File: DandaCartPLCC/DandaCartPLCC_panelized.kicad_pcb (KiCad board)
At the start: 2 copper layers, 93 x 96 mm, 18 parts, among them P1 DAN_CART_EDGE, P2 DAN_CART_EDGE, P3 DAN_CART_EDGE, P4 DAN_CART_EDGE, P5 DAN_CART_EDGE, P6 DAN_CART_EDGE, U1 SST39SF040, U2 SST39SF040, U3 SST39SF040, U4 SST39SF040, U5 SST39SF040, U6 SST39SF040

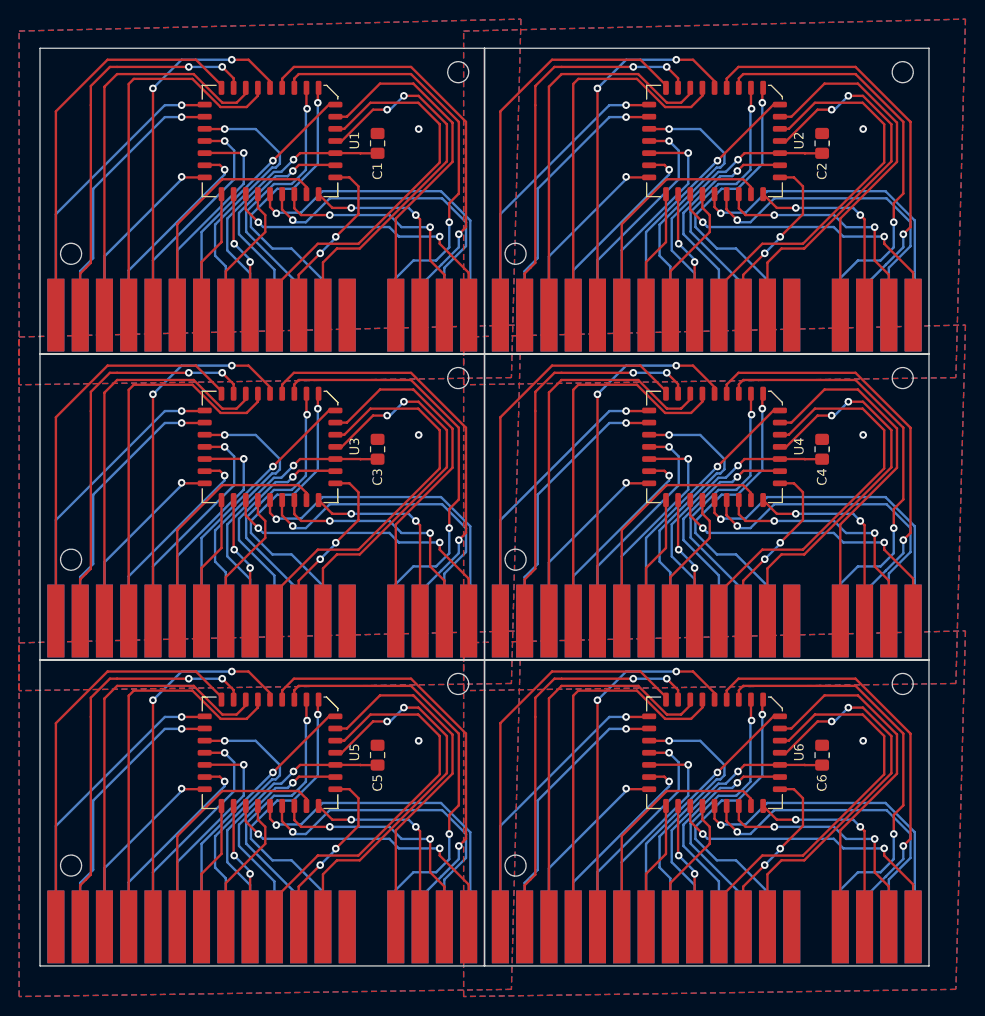
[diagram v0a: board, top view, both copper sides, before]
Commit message: Add files via upload
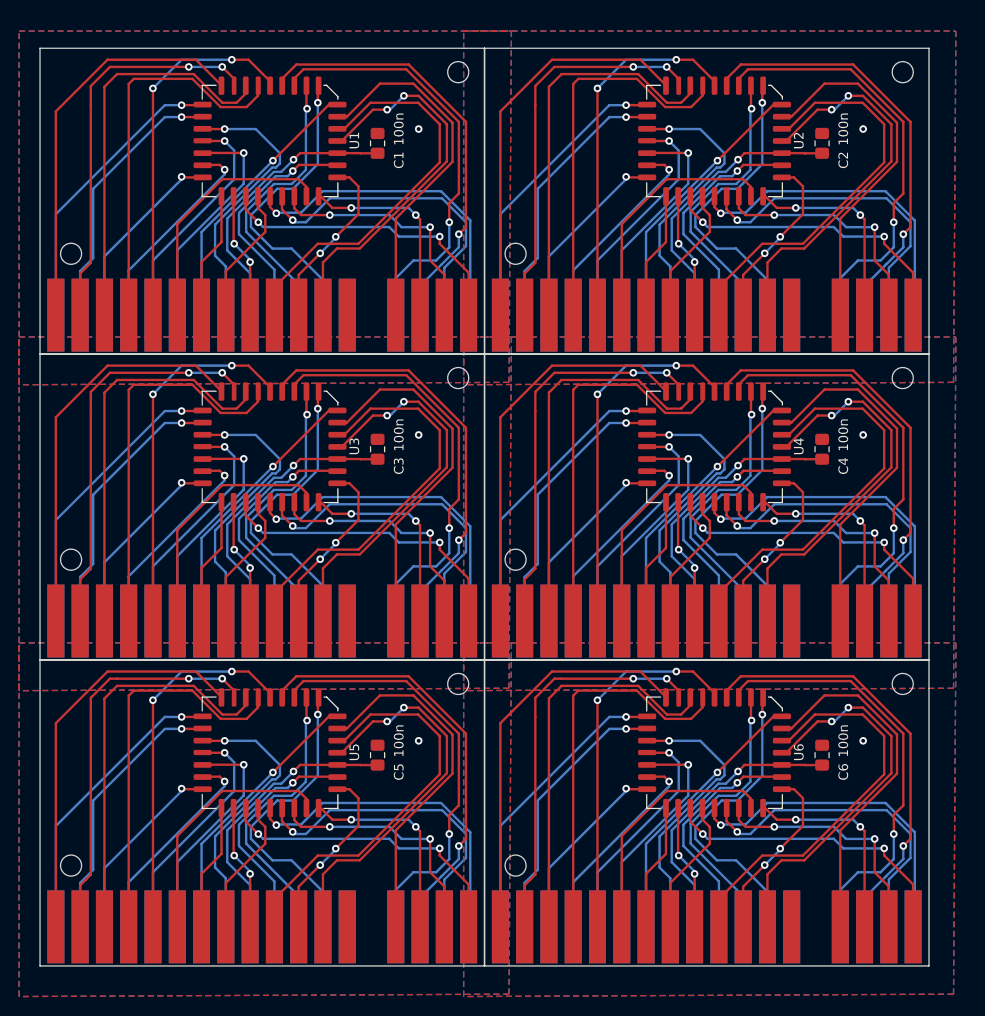
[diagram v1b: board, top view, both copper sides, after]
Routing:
- net A5: track 268.7 -> 271.2 mm
- net D0: track 253.5 -> 251.9 mm
- net D2: track 171.4 -> 170.1 mm
- net A4: track 271.7 -> 272.9 mm
- net D1: track 185.3 -> 184.8 mm
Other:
- board text added: "100n"
